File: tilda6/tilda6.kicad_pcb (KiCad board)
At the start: 2 copper layers, 60 x 23.5 mm, 11 parts, among them J1 Conn_02x05_Odd_Even, J2 Conn_02x02_Odd_Even, J3 Conn_02x02_Odd_Even, J4 Conn_02x05_Odd_Even, P1 USB_C_Plug, SW1 SW_SPDT, SW2 SW_SPST, SW3 SW_SPST, U1 ESP32-S2-MINI-1-N4

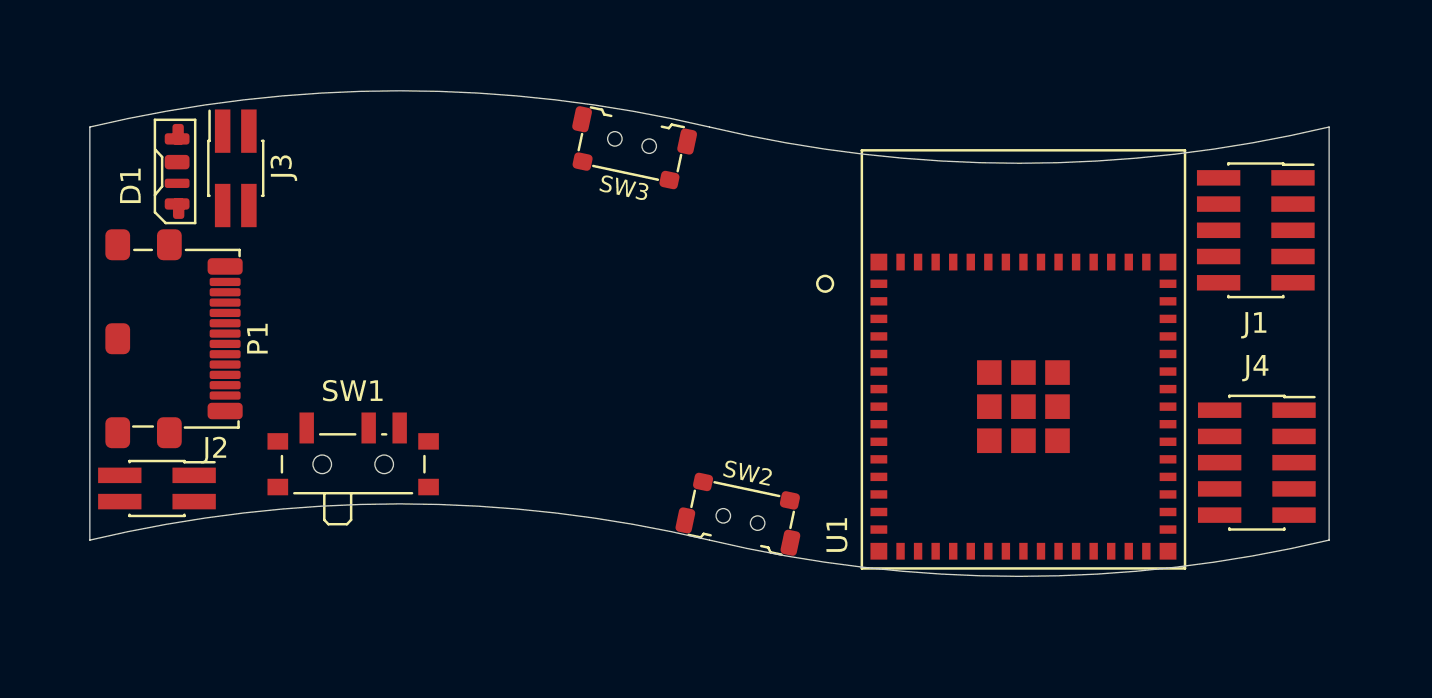
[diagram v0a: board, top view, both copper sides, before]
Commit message: First full layout
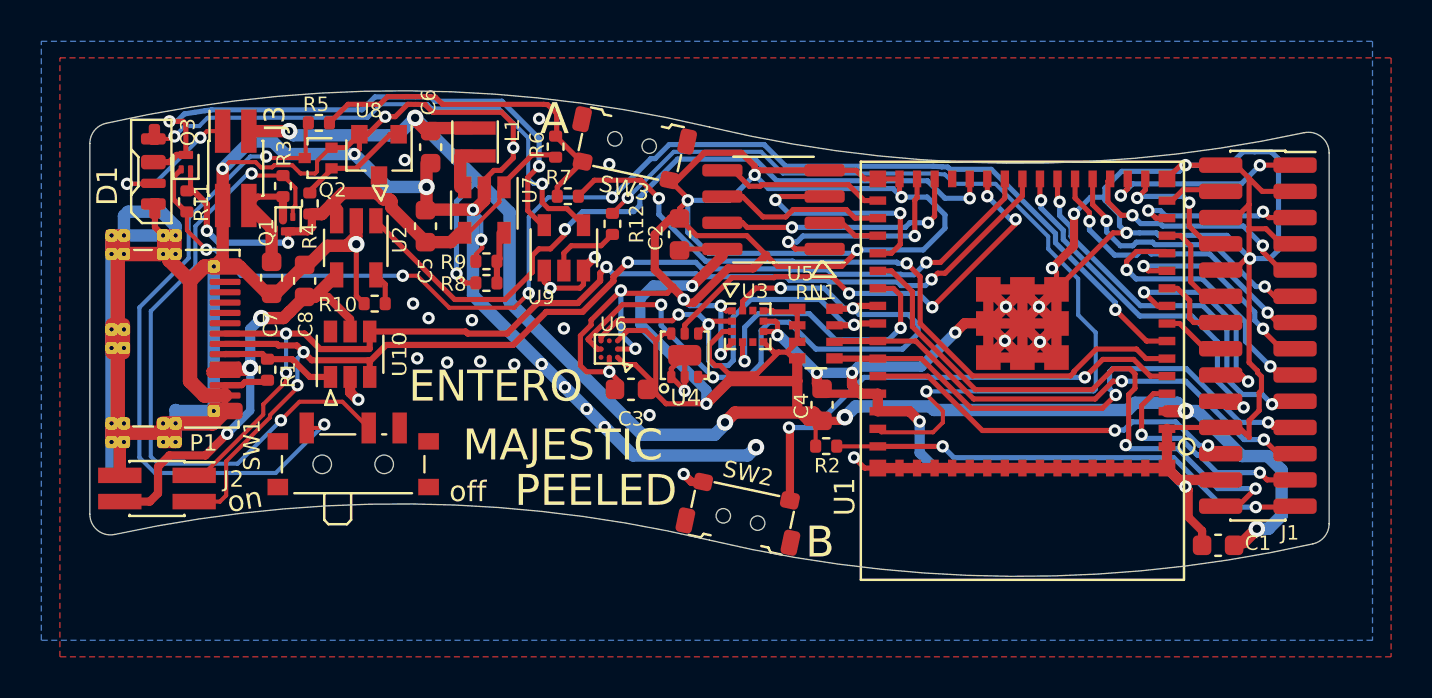
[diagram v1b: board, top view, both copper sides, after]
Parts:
- removed J4: Conn_02x05_Odd_Even, Connector_PinSocket_1.27mm:PinSocket_2x05_P1.27mm_Vertical_SMD
- added C1: C, Capacitor_SMD:C_0603_1608Metric, F.Cu at (154.6, 120.2)
- added C2: C, Capacitor_SMD:C_0603_1608Metric, F.Cu at (128.6, 105.2)
- added C3: C, Capacitor_SMD:C_0603_1608Metric, F.Cu at (126.2, 112.7)
- added C4: C, Capacitor_SMD:C_0603_1608Metric, F.Cu at (135.4, 113.5)
- added C5: C, Capacitor_SMD:C_0603_1608Metric, F.Cu at (116.2, 104.8)
- added C6: C, Capacitor_SMD:C_0603_1608Metric, F.Cu at (116.5, 101.0)
- added C7: C, Capacitor_SMD:C_0603_1608Metric, F.Cu at (108.8, 107.3)
- added C8: C, Capacitor_SMD:C_0603_1608Metric, F.Cu at (110.4, 107.5)
- added L1: MHCHL201610A-2R2M-Q8A, Inductor_SMD:L_Taiyo-Yuden_MD-2020, F.Cu at (118.7, 100.7)
- added Q1: LP0404N3T5G, Package_TO_SOT_SMD:SOT-883, F.Cu at (109.6, 104.7)
- added Q2: 2SK3019, Package_TO_SOT_SMD:SOT-416, F.Cu at (111.0, 101.5)
- added Q3: LP0404N3T5G, Package_TO_SOT_SMD:SOT-883, F.Cu at (104.7, 101.7)
- added R1: 5.1k, Resistor_SMD:R_0402_1005Metric, F.Cu at (108.6, 111.8)
- added R10: 10k, Resistor_SMD:R_0402_1005Metric, F.Cu at (113.8, 108.5)
- added R11: 10k, Resistor_SMD:R_0402_1005Metric, F.Cu at (104.7, 103.6)
- added R12: 1k, Resistor_SMD:R_0402_1005Metric, F.Cu at (125.3, 104.7)
- added R2: 5.1k, Resistor_SMD:R_0402_1005Metric, F.Cu at (135.7, 115.5)
- added R3: 1M, Resistor_SMD:R_0402_1005Metric, F.Cu at (109.3, 102.9)
- added R4: 10k, Resistor_SMD:R_0402_1005Metric, F.Cu at (110.7, 103.7)
- added R5: 10k, Resistor_SMD:R_0402_1005Metric, F.Cu at (111.1, 99.8)
- added R6: 10k, Resistor_SMD:R_0402_1005Metric, F.Cu at (122.5, 101.0)
- added R7: 100k, Resistor_SMD:R_0402_1005Metric, F.Cu at (123.1, 103.3)
- added R8: 267k, Resistor_SMD:R_0402_1005Metric, F.Cu at (119.2, 107.5)
- added R9: 1.43M, Resistor_SMD:R_0402_1005Metric, F.Cu at (119.2, 106.5)
- added RN1: R_Pack04, Resistor_SMD:R_Array_Convex_4x0603, F.Cu at (135.2, 110.0)
- added U10: ESDU5V0H4, Package_TO_SOT_SMD:SOT-23-6, F.Cu at (112.6, 111.0)
- added U2: LTH7R., Package_TO_SOT_SMD:TSOT-23-5, F.Cu at (112.9, 105.8)
- added U3: QMA7981, Package_LGA:LGA-12_2x2mm_P0.5mm, F.Cu at (131.8, 109.7)
- added U4: A1006TL, tilda6:A1006TL, F.Cu at (128.8, 111.0)
- added U5: ESP-PSRAM32, Package_SO:SOIC-8_3.9x4.9mm_P1.27mm, F.Cu at (133.1, 104.0)
- added U6: QMC7983, tilda6:QMC7983, F.Cu at (125.2, 110.8)
- added U7: MT3520B, Package_TO_SOT_SMD:SOT-23-5, F.Cu at (119.1, 104.0)
- added U8: SSP61CC3002MR, Package_TO_SOT_SMD:SOT-23, F.Cu at (114.0, 101.3)
- added U9: SN74LVC1G125DBVR, Package_TO_SOT_SMD:SOT-23-5, F.Cu at (123.0, 105.8)
- D1: value WS2812B -> WS2812B-SIDE-A
- J1: value Conn_02x05_Odd_Even -> Conn_02x14_Odd_Even; footprint Connector_PinSocket_1.27mm:PinSocket_2x05_P1.27mm_Vertical_SMD -> Connector_PinSocket_1.27mm:PinSocket_2x14_P1.27mm_Vertical_SMD
- P1: footprint corelib:UTC009-C -> corelib:UTC009-C-vias
- moved J1 5.10 mm to (156.6, 110.1)
- moved D1 1.15 mm to (103.2, 102.2)
- moved U1 0.55 mm to (145.2, 111.8), turned to 180 degrees
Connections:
- D1 pad 1: Net-(D1-Pad1) -> /VLED
- D1 pad 2: Net-(D1-Pad2) -> /LEDOUT
- D1 pad 3: Net-(D1-Pad3) -> GND
- J1 pad 1: Net-(J1-Pad1) -> /LCD_DC
- J1 pad 10: Net-(J1-Pad10) -> GND
- J1 pad 2: Net-(J1-Pad2) -> GND
- J1 pad 3: Net-(J1-Pad3) -> GND
- J1 pad 4: Net-(J1-Pad4) -> /LCD_DIN
- J1 pad 5: Net-(J1-Pad5) -> /LCD_CS
- J1 pad 6: Net-(J1-Pad6) -> GND
- J1 pad 7: Net-(J1-Pad7) -> GND
- J1 pad 8: Net-(J1-Pad8) -> /LCD_CLK
- J1 pad 9: Net-(J1-Pad9) -> /LCD_RST
- J2 pad 1: Net-(J2-Pad1) -> /D-
- J2 pad 2: Net-(J2-Pad2) -> GND
- J2 pad 3: Net-(J2-Pad3) -> /D+
- J2 pad 4: Net-(J2-Pad4) -> /VBUS
- J3 pad 1: Net-(J3-Pad1) -> /LEDOUT
- J3 pad 2: Net-(J3-Pad2) -> GND
- J3 pad 3: Net-(J3-Pad3) -> /3V3
- J3 pad 4: Net-(J3-Pad4) -> /VBAT_IN
- P1 pad A4: Net-(P1-PadA4) -> /VBUS
- P1 pad A6: Net-(P1-PadA6) -> /D+
- P1 pad A7: Net-(P1-PadA7) -> /D-
- P1 pad B9: Net-(P1-PadA4) -> /VBUS
- SW2 pad 1: Net-(SW2-Pad1) -> /BTN1
- SW2 pad 2: Net-(SW2-Pad2) -> GND
- SW3 pad 2: Net-(SW3-Pad2) -> GND
- U1 pad 10: Net-(U1-Pad10) -> /BTN3
- U1 pad 11: Net-(U1-Pad11) -> /JOYR
- U1 pad 12: Net-(U1-Pad12) -> /JOYL
- U1 pad 13: Net-(U1-Pad13) -> /JOYC
- U1 pad 14: Net-(U1-Pad14) -> /LCD_CS
- U1 pad 15: Net-(U1-Pad15) -> /LCD_DIN
- U1 pad 16: Net-(U1-Pad16) -> /LCD_CLK
- U1 pad 17: Net-(U1-Pad17) -> /LCD_DC
- U1 pad 18: Net-(U1-Pad18) -> /LCD_RST
- U1 pad 19: Net-(U1-Pad19) -> /JOYU
- U1 pad 20: Net-(U1-Pad20) -> /JOYD
- U1 pad 21: Net-(U1-Pad21) -> /G1
- U1 pad 22: Net-(U1-Pad22) -> /G0
- U1 pad 23: Net-(U1-Pad23) -> /D-
- U1 pad 24: Net-(U1-Pad24) -> /D+
- U1 pad 25: Net-(U1-Pad25) -> /AUTH_WKUP
- U1 pad 26: Net-(U1-Pad26) -> /CHARGE_DET
- U1 pad 28: Net-(U1-Pad28) -> /PSRAMHD
- U1 pad 29: Net-(U1-Pad29) -> /PSRAMCS
- U1 pad 3: Net-(U1-Pad3) -> /3V3
- U1 pad 31: Net-(U1-Pad31) -> /PSRAMD
- U1 pad 32: Net-(U1-Pad32) -> /PSRAMCLK
- U1 pad 33: Net-(U1-Pad33) -> /PSRAMQ
- U1 pad 34: Net-(U1-Pad34) -> /PSRAMWP
- U1 pad 35: Net-(U1-Pad35) -> /LCD_PWR_EN
- U1 pad 36: Net-(U1-Pad36) -> /ACCL_INT
- U1 pad 37: Net-(U1-Pad37) -> /SI2C_SCL
- U1 pad 38: Net-(U1-Pad38) -> /SI2C_SDA
- U1 pad 39: Net-(U1-Pad39) -> /PI2C_SCL
- U1 pad 4: Net-(U1-Pad4) -> /IO0
- U1 pad 40: Net-(U1-Pad40) -> /PI2C_SDA
- U1 pad 41: Net-(U1-Pad41) -> /LCD_BL_EN
- U1 pad 44: Net-(U1-Pad44) -> /LEDDATA
- U1 pad 45: Net-(U1-Pad45) -> /EN
- U1 pad 5: Net-(U1-Pad5) -> /BTN1
- U1 pad 6: Net-(U1-Pad6) -> /BTN2
- U1 pad 7: Net-(U1-Pad7) -> /LED_PWR
- U1 pad 8: Net-(U1-Pad8) -> /G2
- U1 pad 9: Net-(U1-Pad9) -> /G3
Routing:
- net GND: track 0.00 -> 405.8 mm, vias 0 -> 55
- net /3V3: track 0.00 -> 125.9 mm, vias 0 -> 9
- net /LED_PWR: track 0.00 -> 62.2 mm, vias 0 -> 5
- net /D+: track 0.00 -> 53.8 mm, vias 0 -> 4
- net /D-: track 0.00 -> 53.4 mm, vias 0 -> 4
- net /LEDDATA: track 0.00 -> 45.9 mm, vias 0 -> 2
- net /CHARGE_DET: track 0.00 -> 35.7 mm, vias 0 -> 2
- net /SI2C_SCL: track 0.00 -> 35.7 mm, vias 0 -> 4
- net /BTN2: track 0.00 -> 35.3 mm, vias 0 -> 2
- net Net-(Q2-Pad3): track 0.00 -> 32.4 mm, vias 0 -> 2
- net Net-(Q1-Pad1): track 0.00 -> 32.1 mm, vias 0 -> 2
- net /LCD_PWR_EN: track 0.00 -> 29.2 mm, vias 0 -> 2
- net /VLED: track 0.00 -> 28.0 mm, vias 0 -> 2
- net /VBAT_SW: track 0.00 -> 27.4 mm, vias 0 -> 2
- net /PI2C_SDA: track 0.00 -> 26.4 mm, vias 0 -> 2
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- added copper zone on B.Cu, net GND
- added copper zone on F.Cu, net GND
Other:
- outline, holes or cut-outs redrawn
- net class Default: clearance 0.2 -> 0.127
- rule trace_clearance: 0.2 -> 0.127
- board text added: "A"
- board text added: "B"
- board text added: "ENTERO"
- board text added: "MAJESTIC"
- board text added: "PEELED"
- board text added: "off"
- board text added: "on"
